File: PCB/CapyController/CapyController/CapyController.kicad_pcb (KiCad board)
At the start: 2 copper layers, 99.8 x 69.8 mm, 48 parts, among them J1 Conn_01x02, J10 Conn_01x04, J11 Conn_01x04, J12 Conn_01x04, J13 Conn_01x04, J14 Conn_01x02, J15 Conn_01x02, J16 Conn_01x04, J17 Conn_01x02, J18 Conn_01x04, J19 Conn_02x04_Top_Bottom, J2 Conn_01x08, J20 Conn_02x05_Top_Bottom, J3 Conn_01x08, J4 Conn_01x04, J5 Conn_01x04, J6 Conn_01x04, J7 Conn_01x04, J8 Conn_01x04, J9 Conn_01x04, U1 ESP32-S3-DEVKITC-1-N8R2, U2 TCA9548APWR

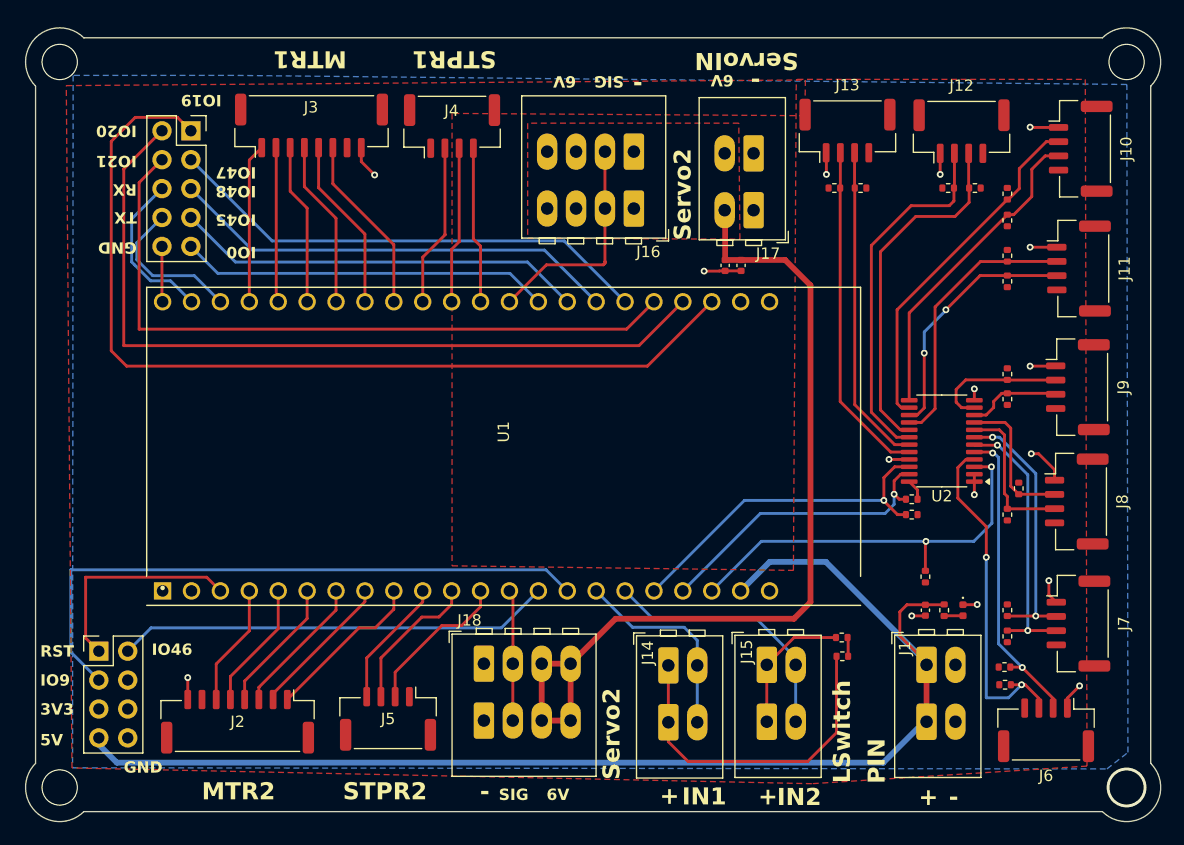
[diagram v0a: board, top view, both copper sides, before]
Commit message: Updated Both PCBs
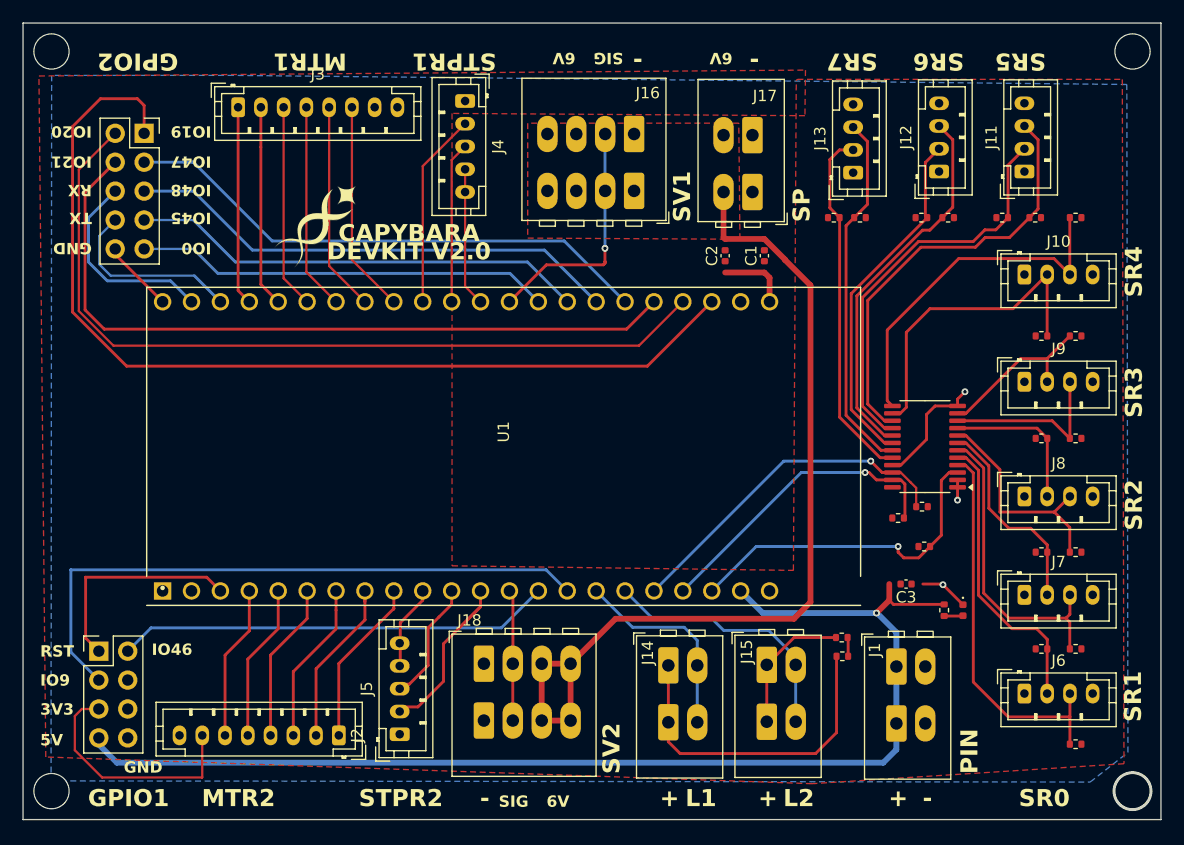
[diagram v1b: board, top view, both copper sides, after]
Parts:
- added G***: LOGO, CapyPower_Footprints:IPRL_Helix_14mm, F.Cu at (151.2, 77.4)
- J10, J11, J12, J13, J6, J7, J8, J9: footprint Connector_JST:JST_GH_BM04B-GHS-TBT_1x04-1MP_P1.25mm_Vertical -> Connector_JST:JST_PH_B4B-PH-K_1x04_P2.00mm_Vertical
- J2, J3: footprint Connector_JST:JST_GH_BM08B-GHS-TBT_1x08-1MP_P1.25mm_Vertical -> Connector_JST:JST_PH_B8B-PH-K_1x08_P2.00mm_Vertical
- J4, J5: footprint Connector_JST:JST_GH_BM04B-GHS-TBT_1x04-1MP_P1.25mm_Vertical -> Connector_JST:JST_PH_B5B-PH-K_1x05_P2.00mm_Vertical
- moved R13 12.9 mm to (215.0, 87.0), turned to 0 degrees
- moved J10 12.1 mm to (213.5, 81.6), turned to 0 degrees
- moved J11 9.78 mm to (213.5, 72.5), turned to 90 degrees
- moved J2 8.98 mm to (153.2, 122.1)
- moved R4 8.11 mm to (218.0, 122.9), turned to 0 degrees
- moved R10 6.92 mm to (218.0, 96.0), turned to 0 degrees
- moved R11 6.87 mm to (218.0, 87.0), turned to 180 degrees
- moved R8 6.85 mm to (218.0, 106.0), turned to 0 degrees
- moved J3 6.65 mm to (144.4, 66.9)
- moved R14 6.11 mm to (214.4, 76.6), turned to 0 degrees
- moved R6 6.10 mm to (218.0, 114.5), turned to 0 degrees
- moved R12 6.01 mm to (218.0, 76.6), turned to 0 degrees
- moved R7 5.92 mm to (215.0, 106.0), turned to 0 degrees
- moved J7 5.38 mm to (213.5, 109.8), turned to 0 degrees
- moved R9 4.83 mm to (215.0, 96.0), turned to 0 degrees
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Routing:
- net +3.3V: track 3.53 -> 23.0 mm
- net /SDA5: track 22.0 -> 38.0 mm, vias 2 -> 0
- net /SCL5: track 24.1 -> 35.3 mm
- net GND: track 38.8 -> 29.4 mm, vias 16 -> 3
- net /SDA3: track 8.29 -> 15.5 mm
- net /RST: track 36.2 -> 29.9 mm, vias 2 -> 1
- net /SDA2: track 13.6 -> 19.5 mm
- net +5V: track 111.2 -> 105.3 mm, vias 0 -> 1
- net /SCL1: track 23.6 -> 18.2 mm, vias 2 -> 0
- net /IO19: track 82.4 -> 86.8 mm
- net /IN1_R: track 13.6 -> 18.0 mm
- net /STPR_PUL2: track 11.3 -> 7.01 mm
- net /IO47: track 43.3 -> 47.4 mm
- net /IO48: track 39.7 -> 43.8 mm
- net /IO45: track 36.1 -> 40.2 mm
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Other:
- board size 99.8 x 69.8 mm -> 100 x 70 mm
- board text added: "CAPYBARA"
- board text added: "DEVKIT V2.0"
- board text added: "Designed by: Ryusei Kinosaki"
- board text added: "GPIO1"
- board text added: "GPIO2"
- board text added: "L1"
- board text added: "L2"
- board text added: "SP"
- board text added: "SR0"
- board text added: "SR1"
- board text added: "SR2"
- board text added: "SR3"
- board text added: "SR4"
- board text added: "SR5"
- board text added: "SR6"
- board text added: "SR7"
- board text added: "SV1"
- board text added: "SV2"
- board text removed: "IN1"
- board text removed: "IN2"
- board text removed: "LSwitch"
- board text removed: "Servo2"
- board text removed: "ServoIN"
